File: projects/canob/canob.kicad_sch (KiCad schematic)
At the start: 45 parts, among them J1 USB_C_Receptacle_USB2.0, J2 5054481071, J4 Conn_01x02, J6 5054481071, U1 STM32G0B1CBT, U2 TPSM53602RDA, U3 TJA1051T-3, U4 TLV493D, Y1 Crystal_GND24_Small

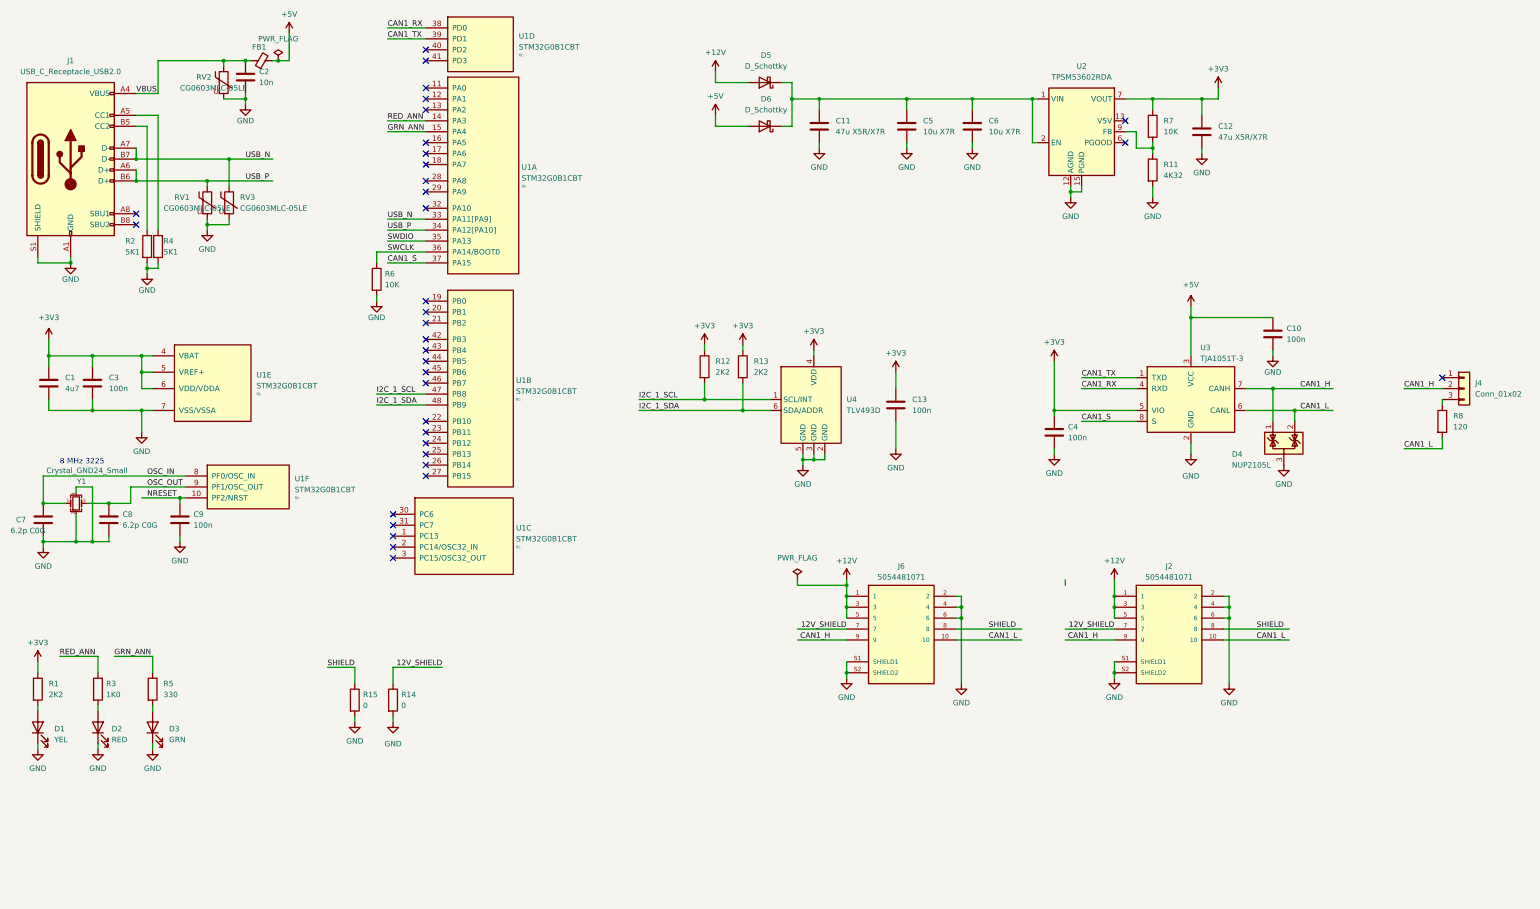
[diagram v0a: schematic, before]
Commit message: wip
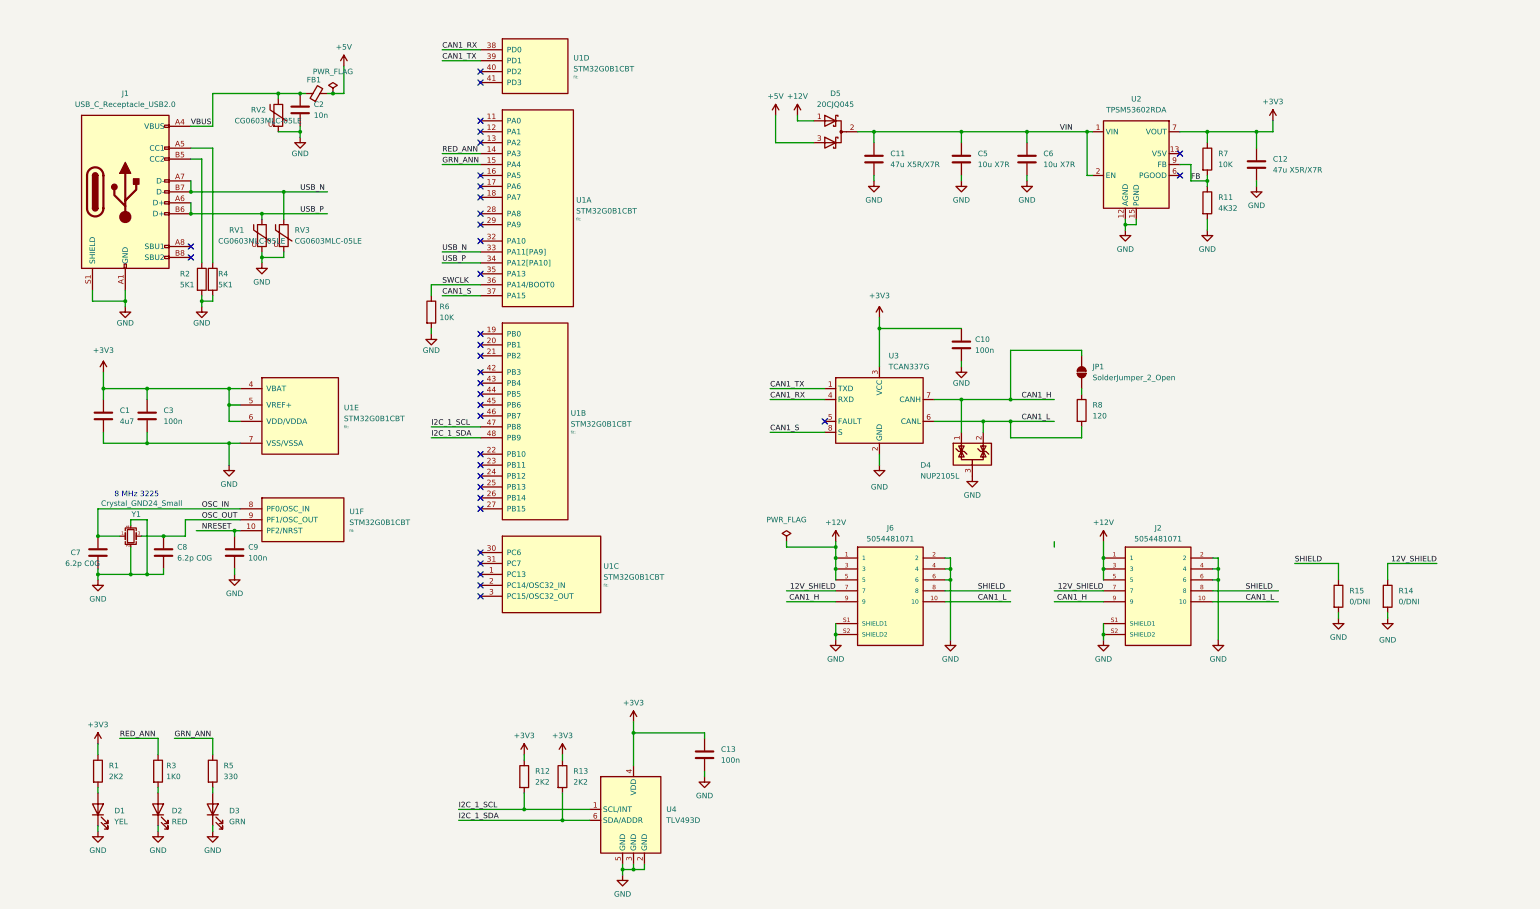
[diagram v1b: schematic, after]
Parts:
- removed C4: 100n, Capacitor_SMD:C_0603_1608Metric, symbol Device:C
- removed D5, D6: D_Schottky, symbol Device:D_Schottky
- removed J4: Conn_01x02, Connector_PinHeader_2.54mm:PinHeader_1x03_P2.54mm_Vertical, symbol Connector_Generic:Conn_01x03
- removed U3: TJA1051T-3, Package_SO:SOIC-8_3.9x4.9mm_P1.27mm, symbol Interface_CAN_LIN:TJA1051T-3
- added D5: 20CJQ045, Package_TO_SOT_SMD:SOT-223-3_TabPin2, symbol Device:D_Schottky_Dual_CommonCathode_AKA_Parallel
- added JP1: SolderJumper_2_Open, Jumper:SolderJumper-2_P1.3mm_Open_TrianglePad1.0x1.5mm, symbol Jumper:SolderJumper_2_Open
- added U3: TCAN337G, Package_TO_SOT_SMD:TSOT-23-8, symbol Interface_CAN_LIN:TCAN337G
- R14, R15: value 0 -> 0/DNI
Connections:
- net +12V: now also D5.1 (A)
- net +3V3: now also C10.1, U3.3 (VCC)
- net +5V: now also D5.3 (A); no longer C10.1
- net CAN1_H: now also JP1.2 (B), U3.7 (CANH)
- net CAN1_L: now also U3.6 (CANL)
- net CAN1_RX: now also U3.4 (RXD)
- net CAN1_S: now also U3.8 (S)
- net CAN1_TX: now also U3.1 (TXD)
- net GND: now also U3.2 (GND)
- net VIN: now reaches C11.1, C5.1, C6.1, U2.1 (VIN), U2.14 (VIN), U2.2 (EN)
- net VIN: now also D5.2 (K)
- net at R8.1: now also JP1.1 (A)
- net FB: now reaches R11.1, R7.2, U2.9 (FB)
- net SWDIO: no longer names the net of U1.35 (PA13)
- no-connect marks 35 -> 36
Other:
- moved on the sheet: C1, C10, C11, C12, C13, C2, C3, C5, C6, C7, C8, C9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
